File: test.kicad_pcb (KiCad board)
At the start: 2 copper layers, 20 x 20 mm, 5 parts, among them U1 STM32F401C_D-E_Ux

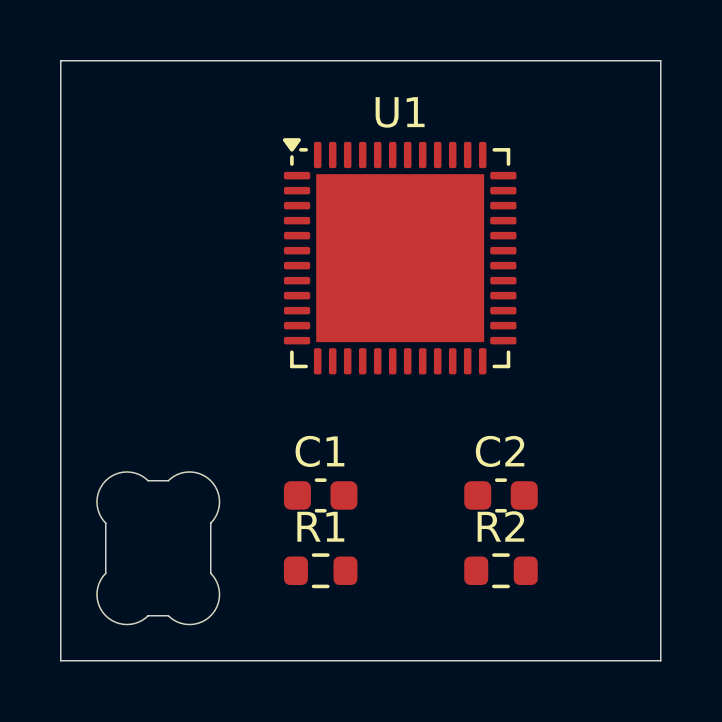
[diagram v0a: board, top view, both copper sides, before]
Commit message: added traces
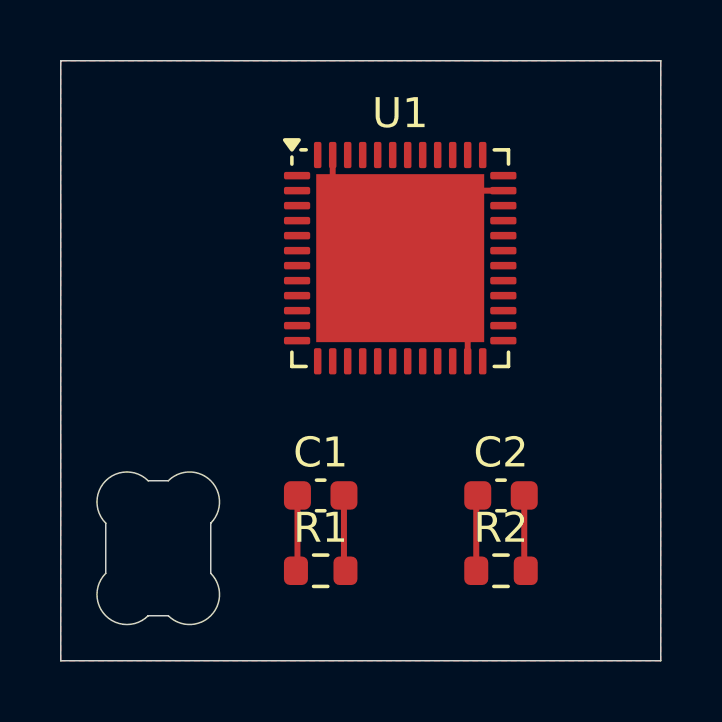
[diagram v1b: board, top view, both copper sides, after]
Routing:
- net Net-(U1-VSS-Pad23): track 0.00 -> 13.1 mm
- net Net-(C2-Pad1): track 0.00 -> 2.53 mm
- net Net-(C2-Pad2): track 0.00 -> 2.53 mm
- net Net-(C1-Pad2): track 0.00 -> 2.53 mm
- net Net-(C1-Pad1): track 0.00 -> 2.53 mm
- added copper zone on F.Cu, net (none)
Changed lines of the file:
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@@
 		(layer "Edge.Cuts")
+	)
+	(segment
+		(start 112.44 83.99)
+		(end 112.44 86.45)
+		(width 0.2)
+		(layer "F.Cu")
+		(net 1)
+	)
+	(segment
+		(start 112.44 86.45)
+		(end 112.49 86.5)
+		(width 0.2)
+		(layer "F.Cu")
+		(net 1)
+	)
+	(segment
+		(start 110.89 86.45)
+		(end 110.84 86.5)
+		(width 0.2)
+		(layer "F.Cu")
+		(net 2)
+	)
+	(segment
+		(start 110.89 83.99)
+		(end 110.89 86.45)
+		(width 0.2)
+		(layer "F.Cu")
+		(net 2)
+	)
+	(segment
+		(start 116.85 84.04)
+		(end 116.9 83.99)
+		(width 0.2)
+		(layer "F.Cu")
+		(net 3)
+	)
+	(segment
+		(start 116.85 86.5)
+		(end 116.85 84.04)
+		(width 0.2)
+		(layer "F.Cu")
+		(net 3)
+	)
+	(segment
+		(start 118.45 86.45)
+		(end 118.5 86.5)
+		(width 0.2)
+		(layer "F.Cu")
+		(net 4)
+	)
+	(segment
+		(start 118.45 83.99)
+		(end 118.45 86.45)
+		(width 0.2)
+		(layer "F.Cu")
+		(net 4)
+	)
+	(segment
+		(start 116.565 78.33)
+		(end 116.565 79.5175)
+		(width 0.2)
+		(layer "F.Cu")
+		(net 15)
+	)
+	(segment
+		(start 114.315 76.08)
+		(end 112.065 73.83)
+		(width 0.2)
+		(layer "F.Cu")
+		(net 15)
+	)
+	(segment
+		(start 112.065 73.83)
+		(end 112.065 72.6425)
+		(width 0.2)
+		(layer "F.Cu")
+		(net 15)
+	)
+	(segment
+		(start 116.565 73.83)
+		(end 117.7525 73.83)
+		(width 0.2)
+		(layer "F.Cu")
+		(net 15)
+	)
+	(segment
+		(start 114.315 76.08)
+		(end 116.565 73.83)
+		(width 0.2)
+		(layer "F.Cu")
+		(net 15)
+	)
+	(segment
+		(start 114.315 76.08)
+		(end 116.565 78.33)
+		(width 0.2)
+		(layer "F.Cu")
+		(net 15)
+	)
+	(zone
+		(net 0)
+		(net_name "")
+		(layer "F.Cu")
+		(hatch edge 0.5)
+		(connect_pads
+			(clearance 0.5)
+		)
+		(min_thickness 0.25)
+		(filled_areas_thickness no)
+		(fill yes
+			(mode hatch)
+			(thermal_gap 0.5)
+			(thermal_bridge_width 0.5)
+			(island_removal_mode 1)
+			(island_area_min 10)
+			(hatch_thickness 1)
+			(hatch_gap 1.5)
+			(hatch_orientation 0)
+			(hatch_border_algorithm hatch_thickness)
+			(hatch_min_hole_area 0.3)
+		)
+		(polygon
+			(pts
+				(xy 103 69.5) (xy 123 69.5) (xy 123 89.5) (xy 103 89.5)
+			)
+		)
 	)
 	(embedded_fonts no)
